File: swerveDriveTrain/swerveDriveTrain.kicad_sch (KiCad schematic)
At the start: 39 parts, among them IC1 TCAN3414DR, J1 RJ45, J2 Screw_Terminal_01x02, J3 Conn_01x06_Pin, J4 S6B-PH-K-S_LF__SN_, U2 Teensy4.0

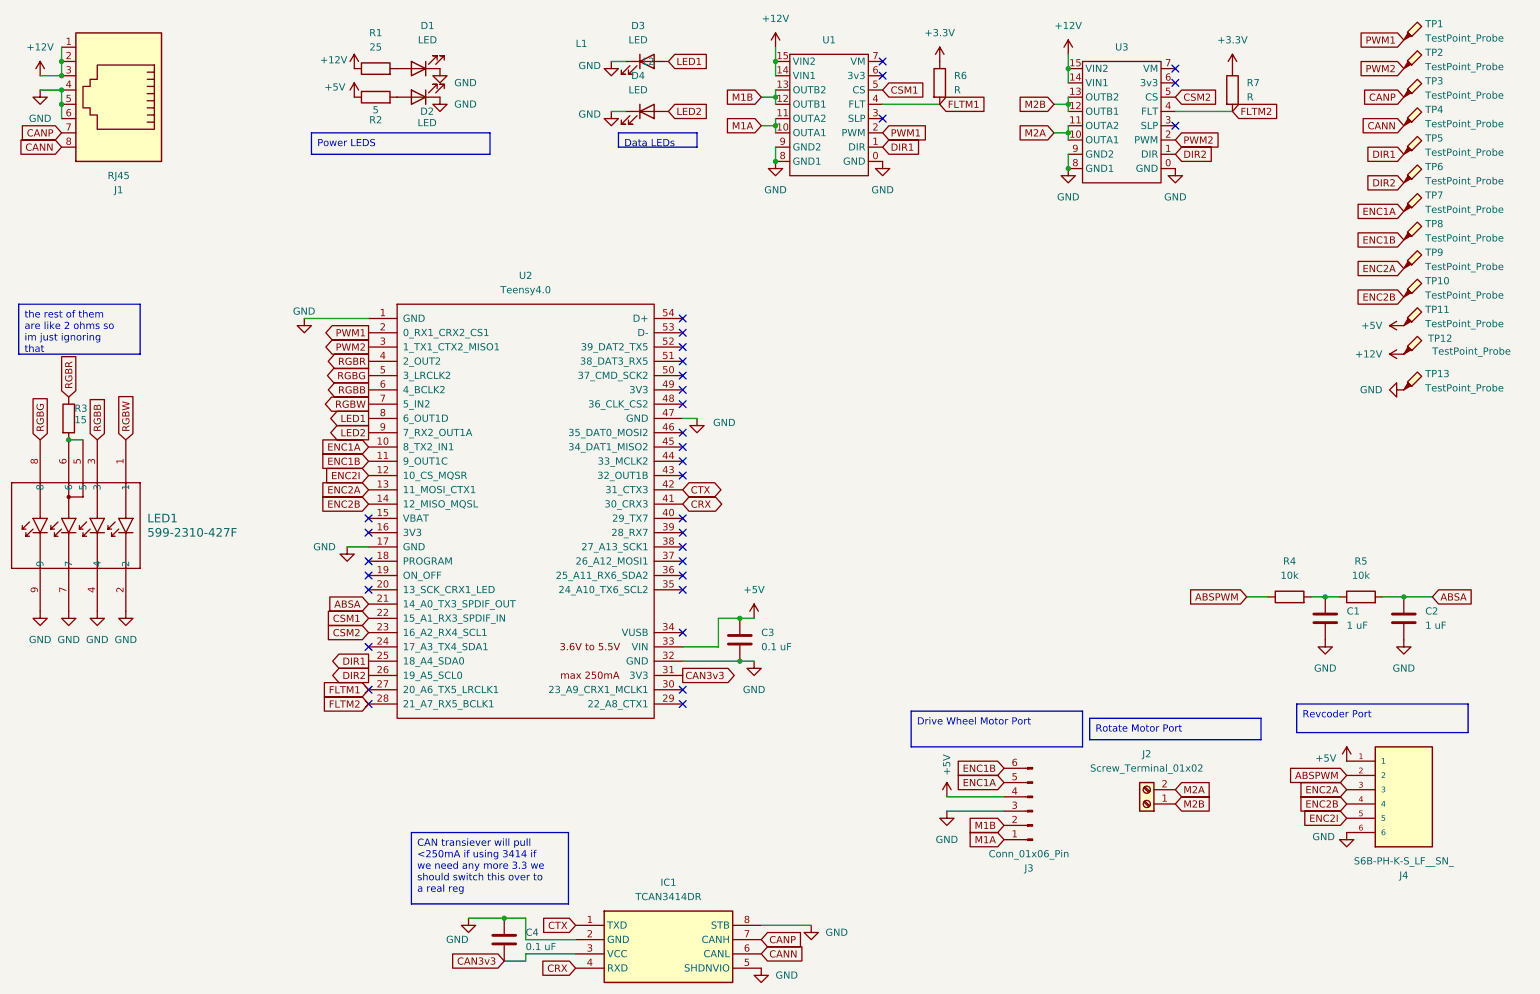
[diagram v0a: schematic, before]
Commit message: new outline
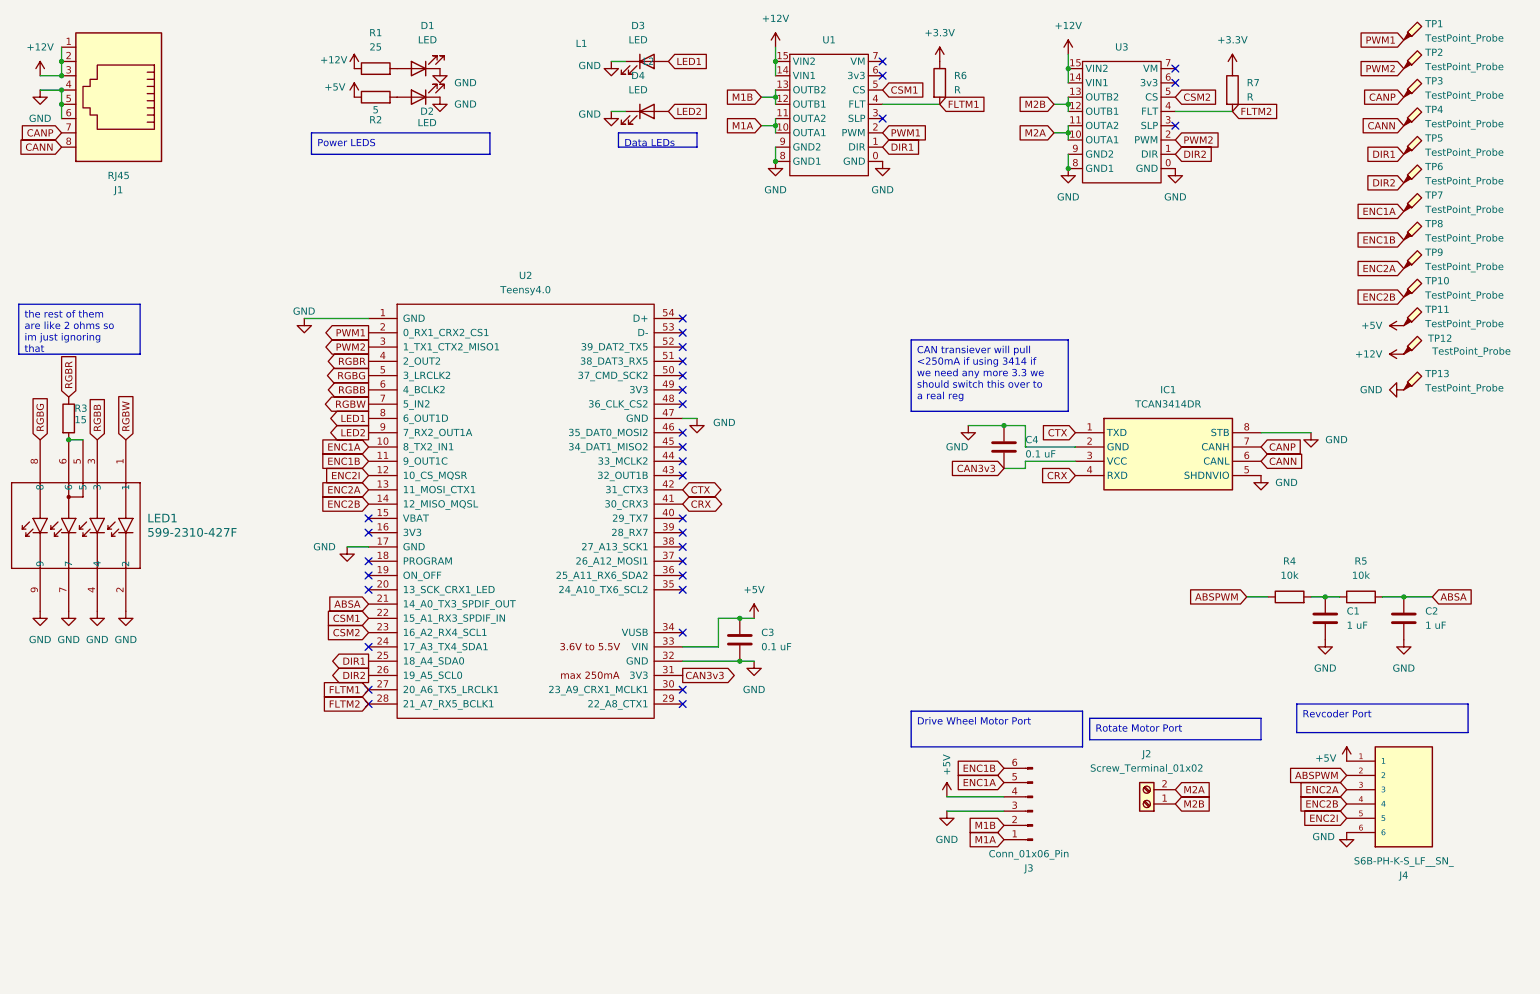
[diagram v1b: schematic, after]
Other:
- moved on the sheet: C4, IC1
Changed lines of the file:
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@@
 	)
 	(junction
-		(at 102.87 173.99)
+		(at 191.77 86.36)
 		(diameter 0)
 		(color 0 0 0 0)
@@
 	(wire
 		(pts
-			(xy 96.52 173.99) (xy 102.87 173.99)
+			(xy 185.42 86.36) (xy 191.77 86.36)
 		)
 		(stroke
@@
 	(wire
 		(pts
-			(xy 157.48 175.26) (xy 148.59 175.26)
+			(xy 246.38 87.63) (xy 237.49 87.63)
 		)
 		(stroke
@@
 	(wire
 		(pts
-			(xy 106.68 177.8) (xy 115.57 177.8)
+			(xy 195.58 90.17) (xy 204.47 90.17)
 		)
 		(stroke
@@
 	(wire
 		(pts
-			(xy 106.68 180.34) (xy 115.57 180.34)
+			(xy 195.58 92.71) (xy 204.47 92.71)
 		)
 		(stroke
@@
 	(wire
 		(pts
-			(xy 106.68 173.99) (xy 106.68 177.8)
+			(xy 195.58 86.36) (xy 195.58 90.17)
 		)
 		(stroke
@@
 	(wire
 		(pts
-			(xy 102.87 181.61) (xy 106.68 181.61)
+			(xy 191.77 93.98) (xy 195.58 93.98)
 		)
 		(stroke
@@
 	(wire
 		(pts
-			(xy 102.87 173.99) (xy 106.68 173.99)
+			(xy 191.77 86.36) (xy 195.58 86.36)
 		)
 		(stroke
@@
 	(wire
 		(pts
-			(xy 106.68 181.61) (xy 106.68 180.34)
+			(xy 195.58 93.98) (xy 195.58 92.71)
 		)
 		(stroke
@@
 	(text_box "CAN transiever will pull <250mA if using 3414 if we need any more 3.3 we should switch this over to a real reg\n"
 		(exclude_from_sim no)
-		(at 86.36 158.75 0)
+		(at 175.26 71.12 0)
 		(size 27.94 12.7)
 		(stroke
@@
 	(global_label "CAN3v3"
 		(shape input)
-		(at 102.87 181.61 180)
+		(at 191.77 93.98 180)
 		(fields_autoplaced yes)
 		(effects
@@
 		)
 		(property "Intersheetrefs" "${INTERSHEET_REFS}"
-			(at 92.8091 181.61 0)
+			(at 181.7091 93.98 0)
 			(effects
 				(font
@@
 	(global_label "CTX"
 		(shape input)
-		(at 115.57 175.26 180)
+		(at 204.47 87.63 180)
 		(fields_autoplaced yes)
 		(effects
@@
 		)
 		(property "Intersheetrefs" "${INTERSHEET_REFS}"
-			(at 109.1377 175.26 0)
+			(at 198.0377 87.63 0)
 			(effects
 				(font
@@
 	(global_label "CRX"
 		(shape input)
-		(at 115.57 182.88 180)
+		(at 204.47 95.25 180)
 		(fields_autoplaced yes)
 		(effects
@@
 		)
 		(property "Intersheetrefs" "${INTERSHEET_REFS}"
-			(at 108.8353 182.88 0)
+			(at 197.7353 95.25 0)
 			(effects
 				(font
@@
 	(global_label "CANP"
 		(shape input)
-		(at 148.59 177.8 0)
+		(at 237.49 90.17 0)
 		(fields_autoplaced yes)
 		(effects
@@
 		)
 		(property "Intersheetrefs" "${INTERSHEET_REFS}"
-			(at 155.8801 177.8 0)
+			(at 244.7801 90.17 0)
 			(effects
 				(font
@@
 	(global_label "CANN"
 		(shape input)
-		(at 148.59 180.34 0)
+		(at 237.49 92.71 0)
 		(fields_autoplaced yes)
 		(effects
@@
 		)
 		(property "Intersheetrefs" "${INTERSHEET_REFS}"
-			(at 155.9406 180.34 0)
+			(at 244.8406 92.71 0)
 			(effects
 				(font
@@
 	(symbol
 		(lib_id "power:GND")
-		(at 157.48 175.26 0)
+		(at 246.38 87.63 0)
 		(unit 1)
 		(exclude_from_sim no)
@@
 		(fields_autoplaced yes)
 		(property "Reference" "#PWR042"
-			(at 157.48 181.61 0)
+			(at 246.38 93.98 0)
 			(effects
 				(font
@@
 		)
 		(property "Value" "GND"
-			(at 160.02 176.5299 0)
+			(at 248.92 88.8999 0)
 			(effects
 				(font
@@
 		)
 		(property "Footprint" ""
-			(at 157.48 175.26 0)
+			(at 246.38 87.63 0)
 			(effects
 				(font
@@
 		)
 		(property "Datasheet" ""
-			(at 157.48 175.26 0)
+			(at 246.38 87.63 0)
 			(effects
 				(font
@@
 		)
 		(property "Description" "Power symbol creates a global label with name \"GND\" , ground"
-			(at 157.48 175.26 0)
+			(at 246.38 87.63 0)
 			(effects
 				(font
@@
 	(symbol
 		(lib_id "TCAN3414DR:TCAN3414DR")
-		(at 115.57 175.26 0)
+		(at 204.47 87.63 0)
 		(unit 1)
 		(exclude_from_sim no)
@@
 		(fields_autoplaced yes)
 		(property "Reference" "IC1"
-			(at 132.08 167.64 0)
+			(at 220.98 80.01 0)
 			(effects
 				(font
@@
 		)
 		(property "Value" "TCAN3414DR"
-			(at 132.08 170.18 0)
+			(at 220.98 82.55 0)
 			(effects
 				(font
@@
 		)
 		(property "Footprint" "footprints:SOIC127P600X175-8N"
-			(at 144.78 270.18 0)
+			(at 233.68 182.55 0)
 			(effects
 				(font
@@
 		)
 		(property "Datasheet" "https://www.ti.com/lit/ds/symlink/tcan3414.pdf?ts=1713723144569&ref_url=https%253A%252F%252Fwww.mouser.ch%252F"
-			(at 144.78 370.18 0)
+			(at 233.68 282.55 0)
 			(effects
 				(font
@@
 		)
 		(property "Description" "3.3-V CAN FD transceiver with shut-down and standby mode"
-			(at 115.57 175.26 0)
+			(at 204.47 87.63 0)
 			(effects
 				(font
@@
 		)
 		(property "Height" "1.75"
-			(at 144.78 570.18 0)
+			(at 233.68 482.55 0)
 			(effects
 				(font
@@
 		)
 		(property "Mouser Part Number" "595-TCAN3414DR"
-			(at 144.78 670.18 0)
+			(at 233.68 582.55 0)
 			(effects
 				(font
@@
 		)
 		(property "Mouser Price/Stock" "https://www.mouser.co.uk/ProductDetail/Texas-Instruments/TCAN3414DR?qs=mELouGlnn3egF2AojRJddw%3D%3D"
-			(at 144.78 770.18 0)
+			(at 233.68 682.55 0)
 			(effects
 				(font
@@
 		)
 		(property "Manufacturer_Name" "Texas Instruments"
-			(at 144.78 870.18 0)
+			(at 233.68 782.55 0)
 			(effects
 				(font
@@
 		)
 		(property "Manufacturer_Part_Number" "TCAN3414DR"
-			(at 144.78 970.18 0)
+			(at 233.68 882.55 0)
 			(effects
 				(font
@@
 	(symbol
 		(lib_id "power:GND")
-		(at 148.59 182.88 0)
+		(at 237.49 95.25 0)
 		(unit 1)
 		(exclude_from_sim no)
@@
 		(fields_autoplaced yes)
 		(property "Reference" "#PWR044"
-			(at 148.59 189.23 0)
+			(at 237.49 101.6 0)
 			(effects
 				(font
@@
 		)
 		(property "Value" "GND"
-			(at 151.13 184.1499 0)
+			(at 240.03 96.5199 0)
 			(effects
 				(font
@@
 		)
 		(property "Footprint" ""
-			(at 148.59 182.88 0)
+			(at 237.49 95.25 0)
 			(effects
 				(font
@@
 		)
 		(property "Datasheet" ""
-			(at 148.59 182.88 0)
+			(at 237.49 95.25 0)
 			(effects
 				(font
@@
 		)
 		(property "Description" "Power symbol creates a global label with name \"GND\" , ground"
-			(at 148.59 182.88 0)
+			(at 237.49 95.25 0)
 			(effects
 				(font
@@
 	(symbol
 		(lib_id "power:GND")
-		(at 96.52 173.99 0)
+		(at 185.42 86.36 0)
 		(unit 1)
 		(exclude_from_sim no)
@@
 		(dnp no)
 		(property "Reference" "#PWR041"
-			(at 96.52 180.34 0)
+			(at 185.42 92.71 0)
 			(effects
 				(font
@@
 		)
 		(property "Value" "GND"
-			(at 96.52 177.8 0)
+			(at 185.42 90.17 0)
 			(effects
 				(font
@@
 		)
 		(property "Footprint" ""
-			(at 96.52 173.99 0)
+			(at 185.42 86.36 0)
 			(effects
 				(font
@@
 		)
 		(property "Datasheet" ""
-			(at 96.52 173.99 0)
+			(at 185.42 86.36 0)
 			(effects
 				(font
@@
 		)
 		(property "Description" "Power symbol creates a global label with name \"GND\" , ground"
-			(at 96.52 173.99 0)
+			(at 185.42 86.36 0)
 			(effects
 				(font
@@
 	(symbol
 		(lib_id "Device:C")
-		(at 102.87 177.8 0)
+		(at 191.77 90.17 0)
 		(unit 1)
 		(exclude_from_sim no)
@@
 		(fields_autoplaced yes)
 		(property "Reference" "C4"
-			(at 106.68 176.5299 0)
+			(at 195.58 88.8999 0)
 			(effects
 				(font
@@
 		)
 		(property "Value" "0.1 uF"
-			(at 106.68 179.0699 0)
+			(at 195.58 91.4399 0)
 			(effects
 				(font
@@
 		)
 		(property "Footprint" "Capacitor_SMD:C_0805_2012Metric"
-			(at 103.8352 181.61 0)
+			(at 192.7352 93.98 0)
 			(effects
 				(font
@@
 		)
 		(property "Datasheet" "~"
-			(at 102.87 177.8 0)
+			(at 191.77 90.17 0)
 			(effects
 				(font
@@
 		)
 		(property "Description" "Unpolarized capacitor"
-			(at 102.87 177.8 0)
+			(at 191.77 90.17 0)
 			(effects
 				(font
